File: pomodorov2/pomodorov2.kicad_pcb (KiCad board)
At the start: 2 copper layers, 26 parts, among them J1 USB_B_Micro, J2 TC2050-IDC, J3 SOICbite, U1 MDBT50Q-1MV2, Y1 32.768kHz, Y1 32MHz, Y2 32.768kHz

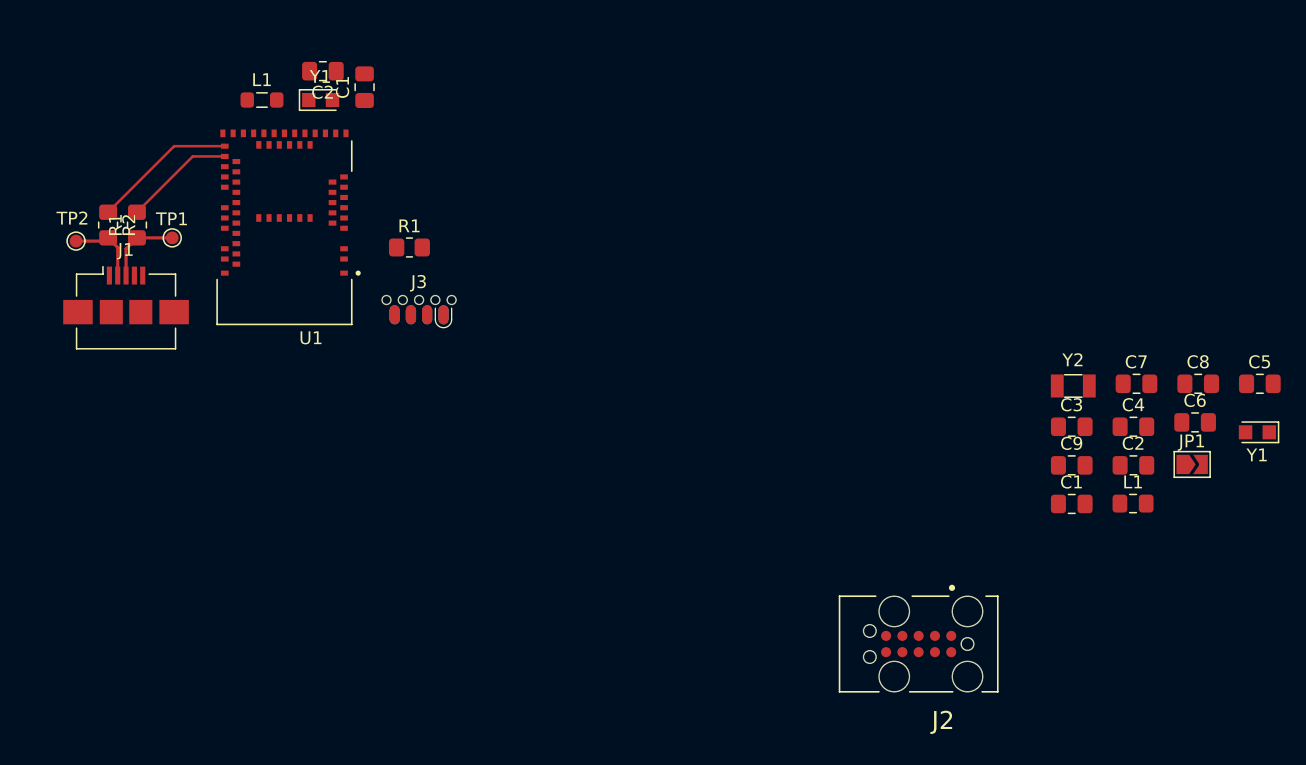
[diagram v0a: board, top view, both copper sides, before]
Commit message: Some layout, schematic work 👷‍♂️
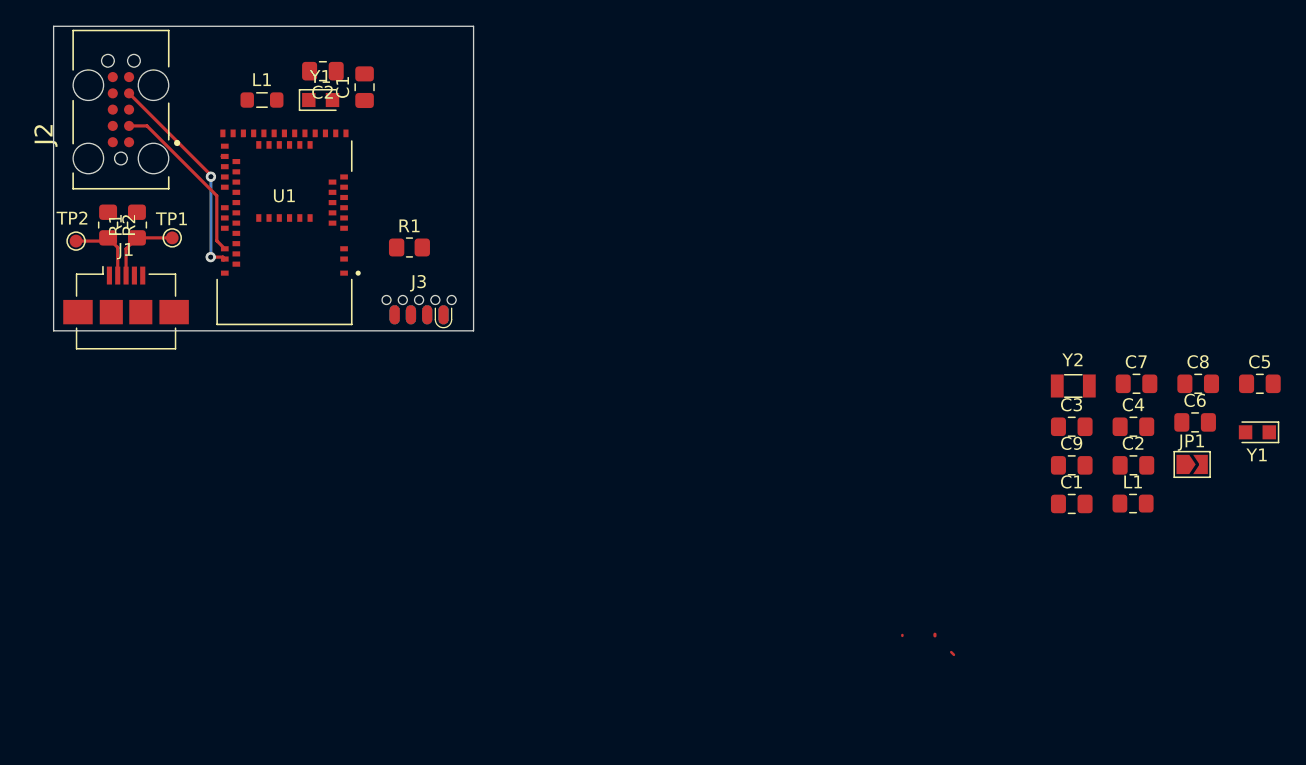
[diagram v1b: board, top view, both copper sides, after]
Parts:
- moved J2 74.9 mm to (94.0, 96.2), turned to 90 degrees
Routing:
- net SWCLK: track 0.07 -> 16.8 mm, vias 0 -> 2
- net SWDIO: track 0.13 -> 13.6 mm
- net USBD-: track 11.2 -> 0.00 mm
- net USBD+: track 8.65 -> 0.25 mm
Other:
- board outline added: 32.8 x 23.8 mm
